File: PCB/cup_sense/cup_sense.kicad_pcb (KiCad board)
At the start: 2 copper layers, 113.8 x 100 mm, 35 parts, among them J1 Connect, J2 Connect, J3 Connect, J4 Connect, J5 Connect, J6 Connect, J7 UPDI, Q1 Q_Photo_NPN, Q2 BC847, Q3 BC847, T1 3Touch, U1 ATtiny816-S

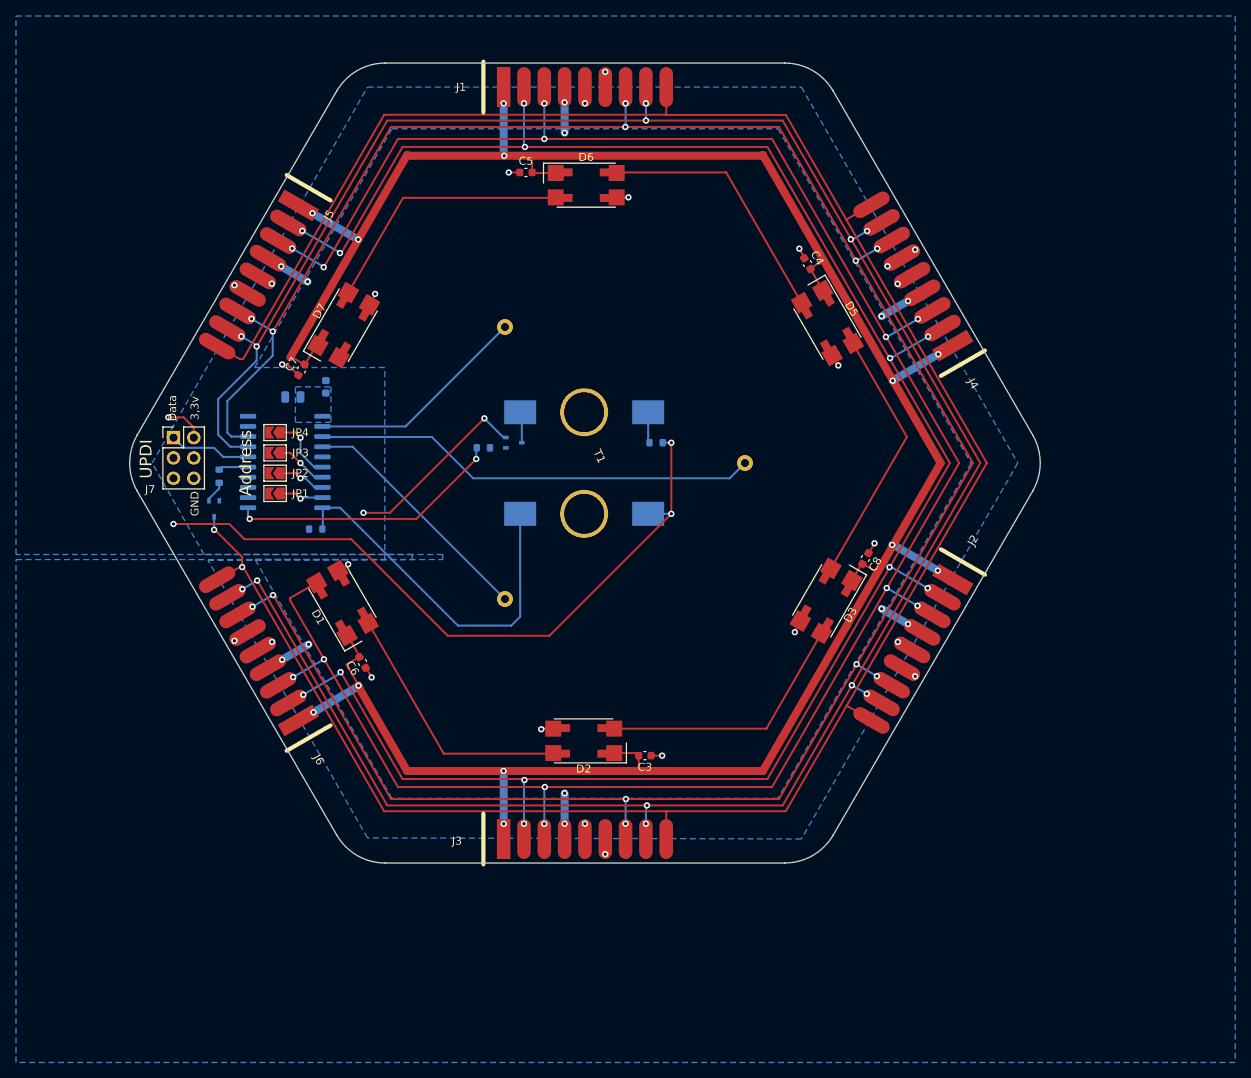
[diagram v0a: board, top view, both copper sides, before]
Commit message: v1.0
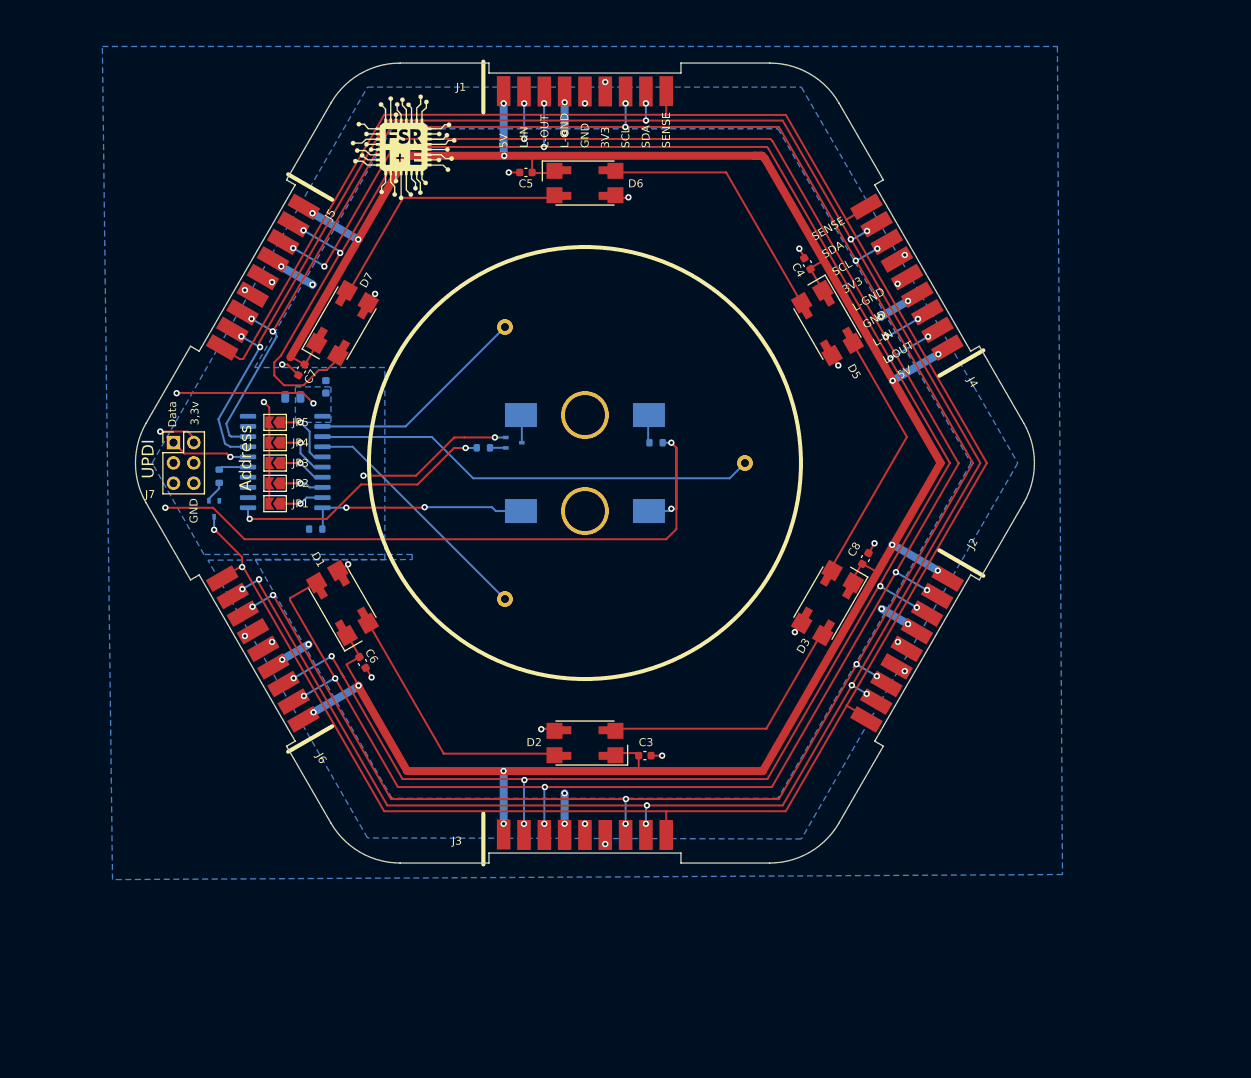
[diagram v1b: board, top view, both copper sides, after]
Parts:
- added G***: LOGO, fsr:FSR_Logo_Small, F.Cu at (-22.7, -39.5)
- added G***: LOGO, fsr:FSR_Logo, B.Cu at (0.00, 25.2)
- added JP5: A4, Jumper:SolderJumper-2_P1.3mm_Open_TrianglePad1.0x1.5mm, F.Cu at (-38.7, -5.08)
- J1, J2, J6: footprint fsr:1x09_EdgeConnect -> fsr:1x09_EdgeConnect_Flip
- moved JP1 1.27 mm to (-38.7, 5.08)
- moved JP2 1.27 mm to (-38.7, 2.54)
- moved JP3 1.27 mm to (-38.7, 0.00)
- moved JP4 1.27 mm to (-38.7, -2.54)
- moved J7 0.61 mm to (-51.4, -2.56)
- moved D4 0.36 mm to (0.00, -6.00)
- moved Q1 0.36 mm to (0.00, 6.00)
- moved D2 0.31 mm to (0.00, 35.0)
- moved D6 0.31 mm to (0.00, -35.0)
- moved D3 0.31 mm to (30.3, 17.5)
- moved D7 0.31 mm to (-30.3, -17.5)
- moved J2 0.23 mm to (40.7, 23.5)
- moved J6 0.22 mm to (-40.7, 23.5)
- moved J5 0.21 mm to (-40.7, -23.5)
- moved J4 0.19 mm to (40.7, -23.5)
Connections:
- J1 pad 2: LED_OUT -> LED_IN
- J1 pad 3: LED_IN -> LED_OUT
- J2 pad 2: LED_OUT -> LED_IN
- J2 pad 3: LED_IN -> LED_OUT
- J6 pad 2: LED_OUT -> LED_IN
- J6 pad 3: LED_IN -> LED_OUT
- U1 pad 5: unconnected-(U1-Pad5) -> Net-(JP5-Pad1)
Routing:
- net LED_OUT: track 246.3 -> 276.4 mm
- net +3V3: track 92.2 -> 111.5 mm, vias 11 -> 12
- net Net-(Q1-Pad2): track 46.8 -> 27.7 mm, vias 0 -> 2
- net GND: track 23.7 -> 32.8 mm, vias 8 -> 9
- net Net-(JP5-Pad1): track 0.00 -> 8.50 mm, vias 0 -> 1
- net Net-(Q2-Pad1): track 0.00 -> 1.99 mm
- net +5V: track 293.2 -> 294.7 mm
- net Net-(JP4-Pad1): track 8.12 -> 7.23 mm
- net GND1: track 41.5 -> 42.4 mm
- net Net-(R2-Pad1): track 34.3 -> 33.6 mm
- net Net-(JP2-Pad1): track 5.93 -> 5.40 mm
- net Net-(JP3-Pad1): track 6.46 -> 5.93 mm
- net UPDI_DATA: track 10.3 -> 10.1 mm, vias 0 -> 1
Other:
- board size 113.8 x 100 mm -> 112.4 x 100 mm
- board text added: "3V3"
- board text added: "5V"
- board text added: "L-GND"
- board text added: "L-IN"
- board text added: "L-OUT"
- board text added: "Panel v1.0"
- board text added: "SCL"
- board text added: "SDA"
- board text added: "SENSE"
- board text removed: "Panel v0.1"
